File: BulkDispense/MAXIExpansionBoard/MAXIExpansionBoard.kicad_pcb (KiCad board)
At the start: 2 copper layers, 57.2 x 100 mm, 30 parts, among them J1 BS1~4, J10 FS3, J11 R6~R7, J12 R8~R9, J13 OS1~4, J14 WV1~2, J15 FS2, J16 FS4, J17 Analog Inputs, J18 Digital IN + R0~R4, J19 Digital Outputs, J2 MV1~4, J20 R4~R9, J21 Flow Sensors, J3 WB/WL, J4 PS/PCV, J5 Screw_Terminal_01x02, J6 R0~R1, J7 R2~R3, J8 R4~R5, J9 FS1

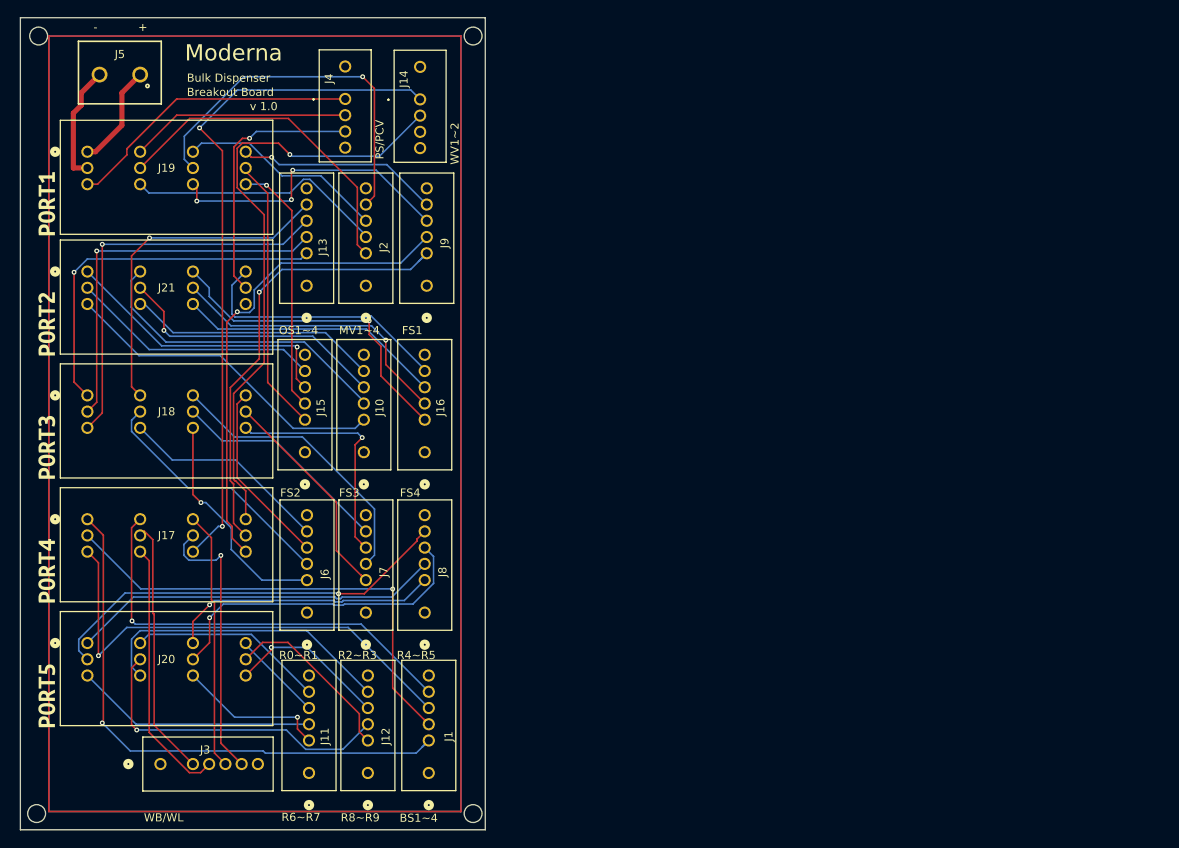
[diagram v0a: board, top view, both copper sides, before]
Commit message: Design Overhaul
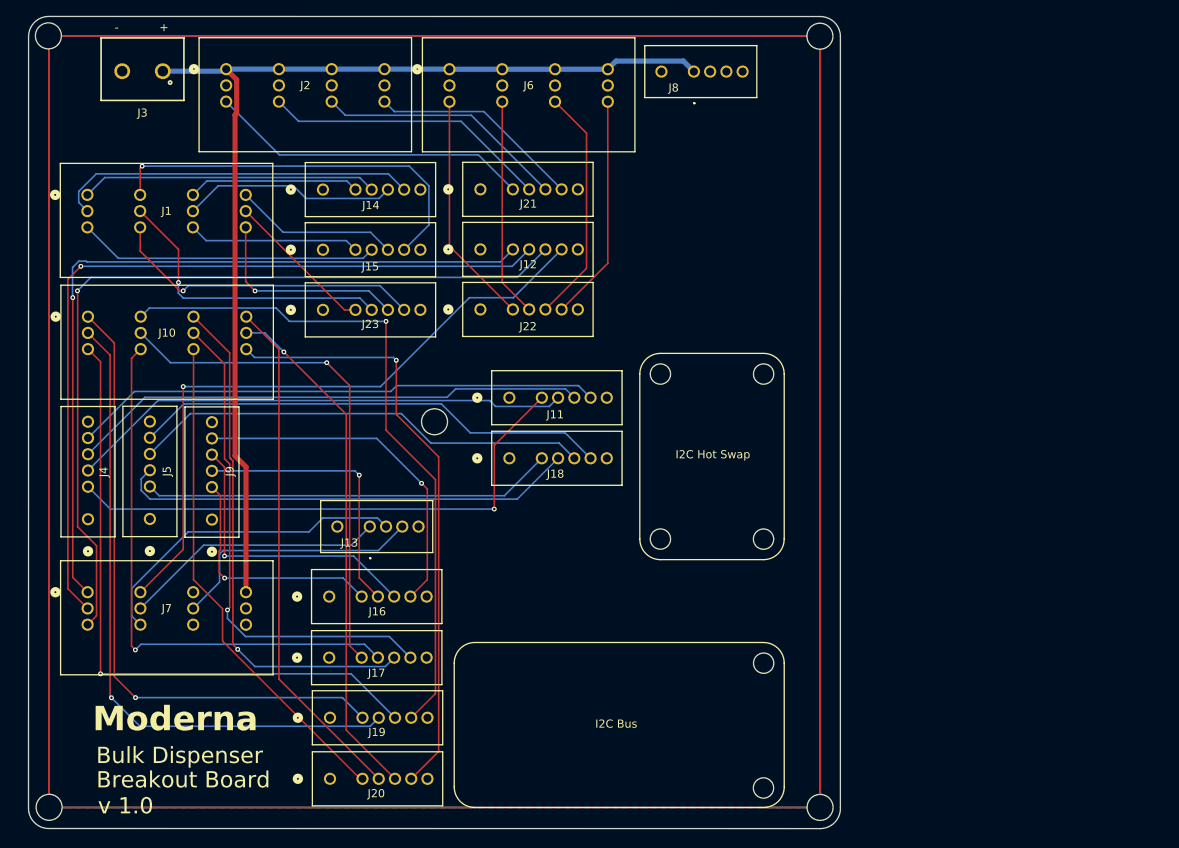
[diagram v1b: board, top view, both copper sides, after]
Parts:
- removed kibuzzard-684C282C: G***, kibuzzard-684C282C
- removed kibuzzard-684C2929: G***, kibuzzard-684C2929
- removed kibuzzard-684C293C: G***, kibuzzard-684C293C
- removed kibuzzard-684C2942: G***, kibuzzard-684C2942
- removed kibuzzard-684C2947: G***, kibuzzard-684C2947
- added H10: MountingHole, MountingHole:MountingHole_2.5mm, F.Cu at (200.6, 84.4)
- added H11: MountingHole, MountingHole:MountingHole_3.2mm_M3, F.Cu at (125.2, 42.7)
- added H5: MountingHole, MountingHole:MountingHole_2.5mm, F.Cu at (213.3, 104.7)
- added H6: MountingHole, MountingHole:MountingHole_2.5mm, F.Cu at (200.6, 104.7)
- added H7: MountingHole, MountingHole:MountingHole_2.5mm, F.Cu at (213.3, 120.0)
- added H8: MountingHole, MountingHole:MountingHole_2.5mm, F.Cu at (213.3, 135.3)
- added H9: MountingHole, MountingHole:MountingHole_2.5mm, F.Cu at (213.3, 84.4)
- added J22: OS1~4, PartsLibrary:CONN_37204-62A3-004PL_3MM, F.Cu at (182.4, 76.4)
- added J23: WB-MV5~6, PartsLibrary:CONN_37204-62A3-004PL_3MM, F.Cu at (163.0, 76.5)
- H1, H2, H3, H4: footprint MountingHole:MountingHole_2.2mm_M2 -> MountingHole:MountingHole_3.2mm_M3
- J1: value BS1~4 -> R0~R5; footprint PartsLibrary:CONN_37204-62A3-004PL_3MM -> PartsLibrary:CONN_37212-62M3-003PL_3MM
- J10: value FS3 -> FS2~FS4; footprint PartsLibrary:CONN_37204-62A3-004PL_3MM -> PartsLibrary:CONN_37212-62M3-003PL_3MM
- J11: value R6~R7 -> MV1~4
- J12: value R8~R9 -> WB/WL
- J13: value OS1~4 -> PS/PCV; footprint PartsLibrary:CONN_37204-62A3-004PL_3MM -> PartsLibrary:3720362A3003PL
- J14: value WV1~2 -> RV1&2; footprint PartsLibrary:3720362A3003PL -> PartsLibrary:CONN_37204-62A3-004PL_3MM
- J15: value FS2 -> RV3&4
- J16: value FS4 -> FS1
- J17: value Analog Inputs -> FS3; footprint PartsLibrary:CONN_37212-62M3-003PL_3MM -> PartsLibrary:CONN_37204-62A3-004PL_3MM
- J18: value Digital IN + R0~R4 -> WB-MV1~4; footprint PartsLibrary:CONN_37212-62M3-003PL_3MM -> PartsLibrary:CONN_37204-62A3-004PL_3MM
- J19: value Digital Outputs -> FS2; footprint PartsLibrary:CONN_37212-62M3-003PL_3MM -> PartsLibrary:CONN_37204-62A3-004PL_3MM
- J2: value MV1~4 -> BS1~4; footprint PartsLibrary:CONN_37204-62A3-004PL_3MM -> PartsLibrary:CONN_37212-62M3-003PL_3MM
- J20: value R4~R9 -> FS4; footprint PartsLibrary:CONN_37212-62M3-003PL_3MM -> PartsLibrary:CONN_37204-62A3-004PL_3MM
- J21: value Flow Sensors -> BS1~4; footprint PartsLibrary:CONN_37212-62M3-003PL_3MM -> PartsLibrary:CONN_37204-62A3-004PL_3MM
- J3: value WB/WL -> Screw_Terminal_01x02; footprint PartsLibrary:CONN_37204-62A3-004PL_3MM -> PartsLibrary:691137710002
- J4: value PS/PCV -> DigitalOUT 0~3; footprint PartsLibrary:3720362A3003PL -> PartsLibrary:CONN_37204-62A3-004PL_3MM
- J5: value Screw_Terminal_01x02 -> DigitalOUT 4~7; footprint PartsLibrary:691137710002 -> PartsLibrary:CONN_37204-62A3-004PL_3MM
- J6: value R0~R1 -> OS1~4; footprint PartsLibrary:CONN_37204-62A3-004PL_3MM -> PartsLibrary:CONN_37212-62M3-003PL_3MM
- J7: value R2~R3 -> AnalogIOs; footprint PartsLibrary:CONN_37204-62A3-004PL_3MM -> PartsLibrary:CONN_37212-62M3-003PL_3MM
- J8: value R4~R5 -> Fan PWR; footprint PartsLibrary:CONN_37204-62A3-004PL_3MM -> PartsLibrary:3720362A3003PL
- moved J3 85.5 mm to (136.8, 47.1), turned to 180 degrees
- moved J1 79.3 mm to (130.0, 62.3), turned to 0 degrees
- moved J19 77.5 mm to (163.9, 126.7)
- moved J8 70.9 mm to (204.7, 47.1), turned to 0 degrees
- moved H1 68.1 mm to (172.8, 90.2)
- moved J6 65.3 mm to (174.6, 46.8), turned to 0 degrees
- moved J12 63.1 mm to (182.4, 69.0), turned to 0 degrees
- moved J4 57.3 mm to (130.1, 98.2), turned to 90 degrees
- moved J18 56.5 mm to (186.0, 94.8)
- moved J21 53.4 mm to (182.4, 61.6)
- moved J11 51.0 mm to (186.0, 87.3), turned to 0 degrees
- moved J5 50.9 mm to (137.7, 98.2), turned to 90 degrees
- moved H4 42.7 mm to (220.2, 137.7)
- moved H3 42.7 mm to (220.2, 42.8)
- moved J9 39.1 mm to (145.3, 98.3)
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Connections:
- J1 pad 1: /AI0 -> /R0_IN
- J1 pad 2: /AI1 -> /R1_IN
- J1 pad 3: /AI2 -> /R2_IN
- J1 pad 4: /AI3 -> /R3_IN
- J1 pad 5: (no net) -> /R4_IN
- J1 pad 6: (no net) -> /R5_IN
- J10 pad 1: /FS3-1 -> /FS2-1
- J10 pad 2: /FS3-2 -> /FS2-2
- J10 pad 3: /FS3-3 -> /FS2-3
- J10 pad 4: /FS3-4 -> /FS2-4
- J10 pad 5: (no net) -> /FS3-1
- J10 pad 6: (no net) -> /FS3-2
- J11 pad 1: /R6_OUT -> /DO0
- J11 pad 2: /R6_IN -> /DO1
- J11 pad 3: /R7_OUT -> /DO2
- J11 pad 4: /R7_IN -> /DO3
- J12 pad 1: /R8_OUT -> /AI4
- J12 pad 2: /R8_IN -> /AI5
- J12 pad 3: /R9_OUT -> /AI6
- J12 pad 4: /R9_IN -> /AI7
- J13 pad 1: /DI0 -> /AI12
- J13 pad 2: /DI1 -> /AI13
- J13 pad 3: /DI2 -> /AO0
- J14 pad 1: /AI8 -> /R0_OUT
- J14 pad 2: /AI9 -> /R0_IN
- J14 pad 3: unconnected-(J14-Pin_3-Pad3) -> /R1_OUT
- J15 pad 1: /FS2-1 -> /R2_OUT
- J15 pad 2: /FS2-2 -> /R2_IN
- J15 pad 3: /FS2-3 -> /R3_OUT
- J15 pad 4: /FS2-4 -> /R3_IN
- J16 pad 1: /FS4-1 -> /FS1-1
- J16 pad 2: /FS4-2 -> /FS1-2
- J16 pad 3: /FS4-3 -> /FS1-3
- J16 pad 4: /FS4-4 -> /FS1-4
- J17 pad 1: /AI0 -> /FS3-1
- J17 pad 2: /AI1 -> /FS3-2
- J17 pad 3: /AI2 -> /FS3-3
- J17 pad 4: /AI3 -> /FS3-4
- J17 pad 5: /AI4 -> (no net)
- J17 pad 6: /AI5 -> (no net)
- J18 pad 1: /DI0 -> /DO4
- J18 pad 2: /DI1 -> /DO5
- J18 pad 3: /DI2 -> /DO6
- J18 pad 4: /DI3 -> /DO7
- J18 pad 5: /R0_IN -> (no net)
- J18 pad 6: /R1_IN -> (no net)
- J19 pad 1: +24V -> /FS2-1
- J19 pad 2: GND -> /FS2-2
- J19 pad 3: /AI12 -> /FS2-3
- J19 pad 4: /AI13 -> /FS2-4
- J19 pad 5: /DO0 -> (no net)
- J19 pad 6: /DO1 -> (no net)
- J2 pad 1: /DO0 -> +24V
- J2 pad 2: /DO1 -> GND
- J2 pad 3: /DO2 -> /AI0
- J2 pad 4: /DO3 -> +24V
- J2 pad 5: (no net) -> GND
- J2 pad 6: (no net) -> /AI1
- J20 pad 1: /R4_IN -> /FS4-1
- J20 pad 2: /R5_IN -> /FS4-2
- J20 pad 3: /R6_IN -> /FS4-3
- J20 pad 4: /R7_IN -> /FS4-4
- J20 pad 5: /R8_IN -> (no net)
- J20 pad 6: /R9_IN -> (no net)
- J21 pad 1: /FS2-3 -> /AI0
- J21 pad 2: /FS2-4 -> /AI1
- J21 pad 3: /FS3-1 -> /AI2
- J21 pad 4: /FS3-2 -> /AI3
- J21 pad 5: /FS3-3 -> (no net)
- J21 pad 6: /FS3-4 -> (no net)
- J3 pad 1: /AI4 -> +24V
- J3 pad 2: /AI5 -> GND
- J4 pad 1: /AI12 -> /DO0
- J4 pad 2: /AI13 -> /DO1
- J4 pad 3: /AO0 -> /DO2
- J5 pad 1: +24V -> /DO4
- J5 pad 2: GND -> /DO5
- J6 pad 1: /R0_OUT -> +24V
- J6 pad 2: /R0_IN -> GND
- J6 pad 3: /R1_OUT -> /DI0
- J6 pad 4: /R1_IN -> +24V
- J6 pad 5: (no net) -> GND
- J6 pad 6: (no net) -> /DI1
- J7 pad 1: /R2_OUT -> /AI4
- J7 pad 2: /R2_IN -> /AI5
- J7 pad 3: /R3_OUT -> /AI6
- J7 pad 4: /R3_IN -> /AI7
- J7 pad 5: (no net) -> /AI12
- J7 pad 6: (no net) -> /AI13
- J8 pad 1: /R4_OUT -> +24V
- J8 pad 2: /R4_IN -> /R6_OUT
- J8 pad 3: /R5_OUT -> unconnected-(J8-Pin_3-Pad3)
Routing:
- net +24V: track 12.8 -> 132.0 mm
- net /AI8: track 84.7 -> 0.00 mm, vias 2 -> 0
- net /AI9: track 74.8 -> 0.00 mm, vias 1 -> 0
- net /AI6: track 31.8 -> 102.3 mm, vias 0 -> 1
- net /AI5: track 32.6 -> 99.9 mm, vias 0 -> 1
- net /AI4: track 32.1 -> 96.0 mm, vias 0 -> 1
- net /DO7: track 0.00 -> 58.8 mm
- net /DO5: track 0.00 -> 56.8 mm
- net /DO6: track 0.00 -> 56.6 mm
- net /FS2-4: track 31.0 -> 83.9 mm, vias 0 -> 1
- net /DO4: track 0.00 -> 50.6 mm
- net /FS2-2: track 32.3 -> 80.9 mm
- net /AI7: track 34.7 -> 81.1 mm
- net /FS2-1: track 34.3 -> 78.3 mm, vias 0 -> 1
- net /FS2-3: track 35.9 -> 79.1 mm
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- added copper zone on B.Cu, net GND
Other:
- board size 57.2 x 100 mm -> 100 x 100 mm
- board text added: "I2C Bus"
- board text added: "I2C Hot Swap"

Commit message: Add latest design
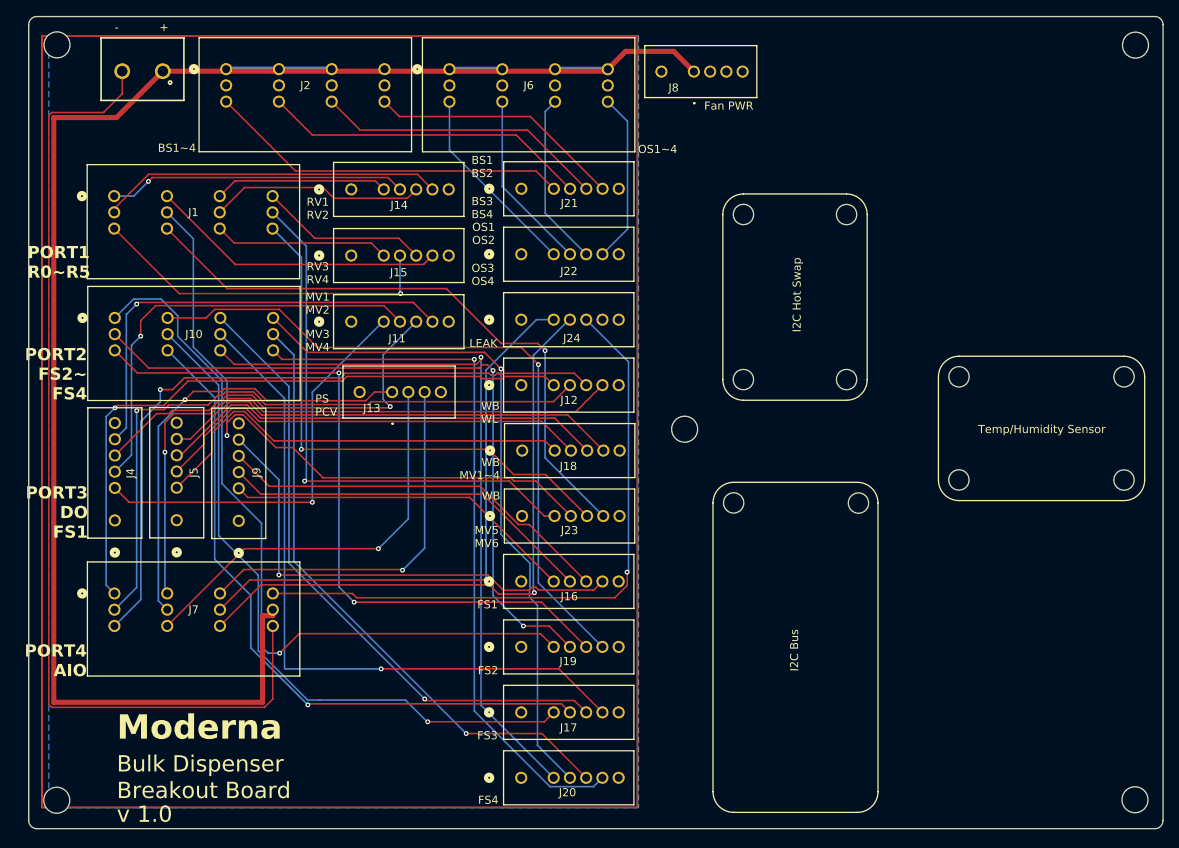
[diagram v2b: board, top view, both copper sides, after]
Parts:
- added H10: MountingHole, MountingHole:MountingHole_2.5mm, F.Cu at (223.5, 85.1)
- added H5: MountingHole, MountingHole:MountingHole_2.5mm, F.Cu at (210.8, 64.7)
- added H6: MountingHole, MountingHole:MountingHole_2.5mm, F.Cu at (223.5, 64.7)
- added H9: MountingHole, MountingHole:MountingHole_2.5mm, F.Cu at (210.8, 85.1)
- added J24: LDS, PartsLibrary:CONN_37204-62A3-004PL_3MM, F.Cu at (187.4, 77.7)
- J13, J8: footprint PartsLibrary:3720362A3003PL -> PartsLibrary:CONN_37203-62A3-003PL_3MM
- moved H13 57.1 mm to (257.7, 84.7), turned to 90 degrees
- moved H15 46.3 mm to (257.7, 97.4), turned to 90 degrees
- moved H12 41.8 mm to (237.3, 84.7), turned to 90 degrees
- moved H3 38.9 mm to (259.1, 43.9)
- moved H4 38.8 mm to (259.0, 136.8)
- moved H8 37.0 mm to (225.0, 100.3), turned to -90 degrees
- moved J23 35.3 mm to (187.5, 101.9)
- moved H1 30.8 mm to (203.6, 91.2)
- moved H14 25.1 mm to (237.3, 97.4), turned to 90 degrees
- moved J19 25.1 mm to (187.4, 118.0)
- moved J17 24.6 mm to (187.4, 126.0)
- moved J16 23.7 mm to (187.4, 109.9)
- moved J20 23.5 mm to (187.4, 134.1)
- moved J11 21.6 mm to (166.5, 77.9)
- moved H7 20.1 mm to (209.6, 100.2), turned to -90 degrees
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- renumbered H6 to H12, H10 to H13, H5 to H14, H9 to H15
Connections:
- J7 pad 10: +24V -> /LDS
- J7 pad 11: unconnected-(J7-Pin_11-Pad11) -> +24V
- J7 pad 7: unconnected-(J7-Pin_7-Pad7) -> /AO0
- J7 pad 8: /AO0 -> /LDS-5V
- J7 pad 9: unconnected-(J7-Pin_9-Pad9) -> /LDS-GND
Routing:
- net GND: track 0.00 -> 122.6 mm
- net +24V: track 132.0 -> 220.9 mm
- net /LDS: track 0.00 -> 79.4 mm, vias 0 -> 1
- net /LDS-GND: track 0.00 -> 76.9 mm, vias 0 -> 1
- net /LDS-5V: track 0.00 -> 71.0 mm, vias 0 -> 1
- net /R4_OUT: track 18.5 -> 67.4 mm, vias 0 -> 1
- net /R4_IN: track 36.7 -> 80.0 mm
- net /R5_OUT: track 25.6 -> 67.2 mm
- net /R5_IN: track 39.0 -> 76.1 mm
- net /FS4-1: track 61.7 -> 88.9 mm, vias 0 -> 1
- net /FS3-4: track 61.6 -> 85.8 mm
- net /AI12: track 32.4 -> 54.9 mm, vias 0 -> 1
- net /FS3-1: track 62.5 -> 84.1 mm
- net /FS4-2: track 63.7 -> 84.6 mm, vias 0 -> 1
- net /AI5: track 99.9 -> 82.4 mm
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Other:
- board size 100 x 100 mm -> 139.7 x 100 mm
- board text added: "BS1 BS2"
- board text added: "BS1~4"
- board text added: "BS3 BS4"
- board text added: "FS1"
- board text added: "FS2"
- board text added: "FS3"
- board text added: "FS4"
- board text added: "Fan PWR"
- board text added: "LEAK"
- board text added: "MV1 MV2"
- board text added: "MV3 MV4"
- board text added: "MV5 MV6"
- board text added: "OS1 OS2"
- board text added: "OS1~4"
- board text added: "OS3 OS4"
- board text added: "PORT1 R0~R5"
- board text added: "PORT2 FS2~ FS4"
- board text added: "PORT3 DO FS1"
- board text added: "PORT4 AIO"
- board text added: "PS PCV"
- board text added: "RV1 RV2"
- board text added: "RV3 RV4"
- board text added: "Temp/Humidity Sensor"
- board text added: "WB"
- board text added: "WB MV1~4"
- board text added: "WB WL"
